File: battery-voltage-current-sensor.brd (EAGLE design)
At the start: 100 x 80 mm, 0 parts

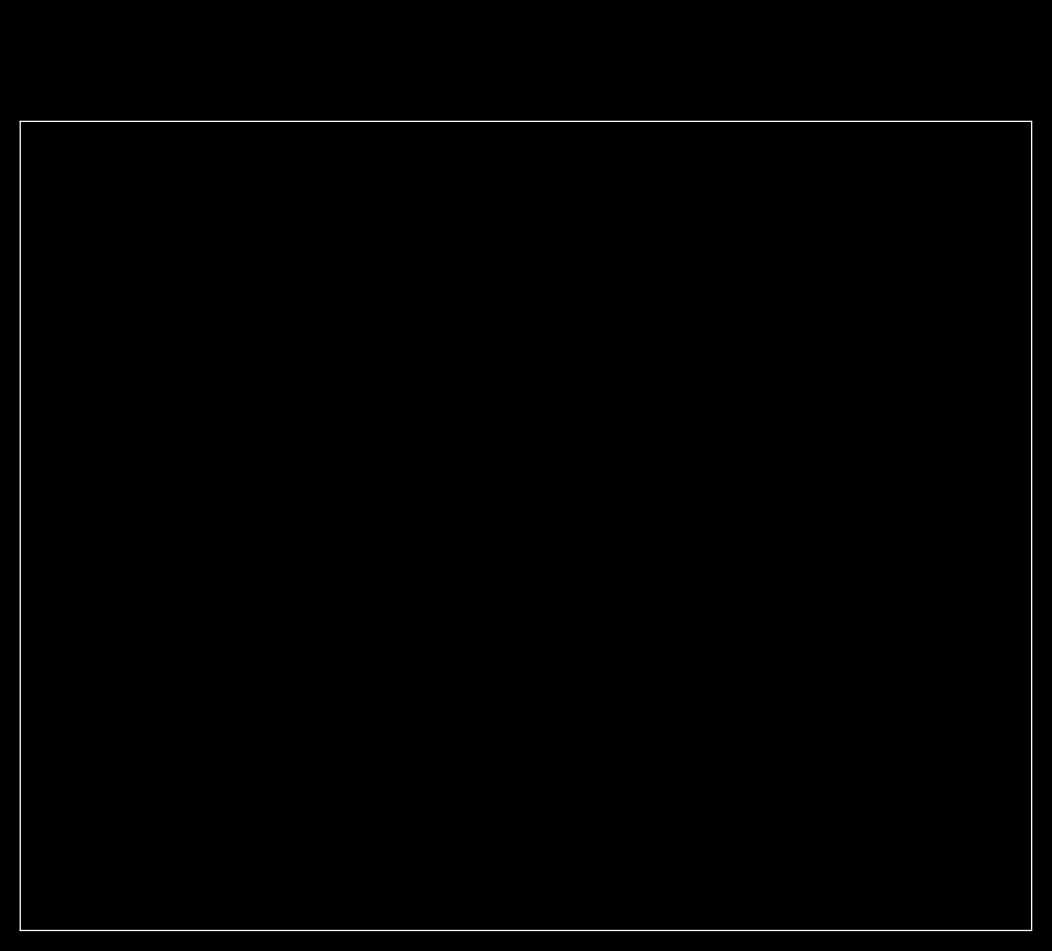
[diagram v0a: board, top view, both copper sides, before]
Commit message: DCDC added
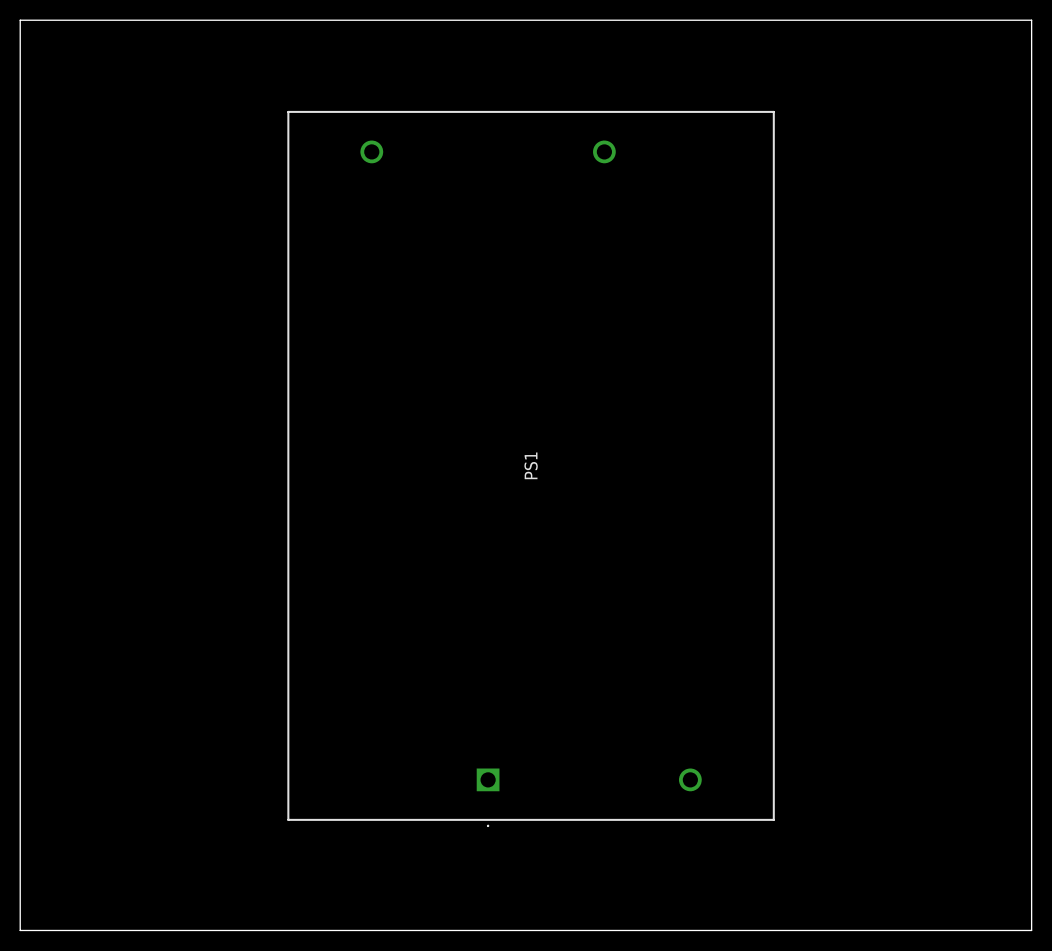
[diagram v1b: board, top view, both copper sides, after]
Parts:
- added PS1: PV15-27B12R3, SamacSys_Parts:PV1527B12R3
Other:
- board size 100 x 80 mm -> 100 x 90 mm
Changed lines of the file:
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@@
 <setting verticaltext="up"/>
 </settings>
-<grid distance="50" unitdist="mil" unit="mil" style="lines" multiple="1" display="no" altdistance="5" altunitdist="mil" altunit="mil"/>
+<grid distance="1" unitdist="mm" unit="mm" style="lines" multiple="1" display="no" altdistance="5" altunitdist="mil" altunit="mil"/>
 <layers>
 <layer number="1" name="Top" color="4" fill="1" visible="yes" active="yes"/>
@@
 <plain>
 <wire x1="0" y1="0" x2="100" y2="0" width="0" layer="20"/>
-<wire x1="100" y1="0" x2="100" y2="80" width="0" layer="20"/>
-<wire x1="100" y1="80" x2="0" y2="80" width="0" layer="20"/>
-<wire x1="0" y1="80" x2="0" y2="0" width="0" layer="20"/>
+<wire x1="100" y1="0" x2="100" y2="90" width="0" layer="20"/>
+<wire x1="100" y1="90" x2="0" y2="90" width="0" layer="20"/>
+<wire x1="0" y1="90" x2="0" y2="0" width="0" layer="20"/>
 </plain>
 <attributes>
@@
 </autorouter>
 <elements>
+<element name="PS1" library="SamacSys_Parts" package="PV1527B12R3" value="PV15-27B12R3" x="46.26" y="14.89" smashed="yes" rot="R90">
+<attribute name="DESCRIPTION" value="Isolated Module DC DC Converter 1 Output 12V 1.25A 100V - 1000V Input" x="76.74" y="94.9" size="1.778" layer="27" rot="R90" display="off"/>
+<attribute name="HEIGHT" value="24mm" x="76.74" y="94.9" size="1.778" layer="27" rot="R90" display="off"/>
+<attribute name="MANUFACTURER_NAME" value="Mornsun Power" x="76.74" y="94.9" size="1.778" layer="27" rot="R90" display="off"/>
+<attribute name="MANUFACTURER_PART_NUMBER" value="PV15-27B12R3" x="76.74" y="94.9" size="1.778" layer="27" rot="R90" display="off"/>
+<attribute name="MOUSER_PART_NUMBER" value="" x="76.74" y="94.9" size="1.778" layer="27" rot="R90" display="off"/>
+<attribute name="MOUSER_PRICE-STOCK" value="" x="76.74" y="94.9" size="1.778" layer="27" rot="R90" display="off"/>
+<attribute name="NAME" x="50.51" y="45.935" size="1.27" layer="25" rot="R90" align="center"/>
+<attribute name="VALUE" x="50.51" y="45.935" size="1.27" layer="27" rot="R90" align="center"/>
+</element>
 </elements>
 <signals>
